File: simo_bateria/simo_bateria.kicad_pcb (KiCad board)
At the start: 2 copper layers, 65 x 35 mm, 16 parts, among them J1 BAT_LEVEL, J2 Plugin, J3 VBAT IN, J4 SWD, SW1 SW_Reed, U1 mod_mt3608, U2 BSS314PEH6327XTSA1

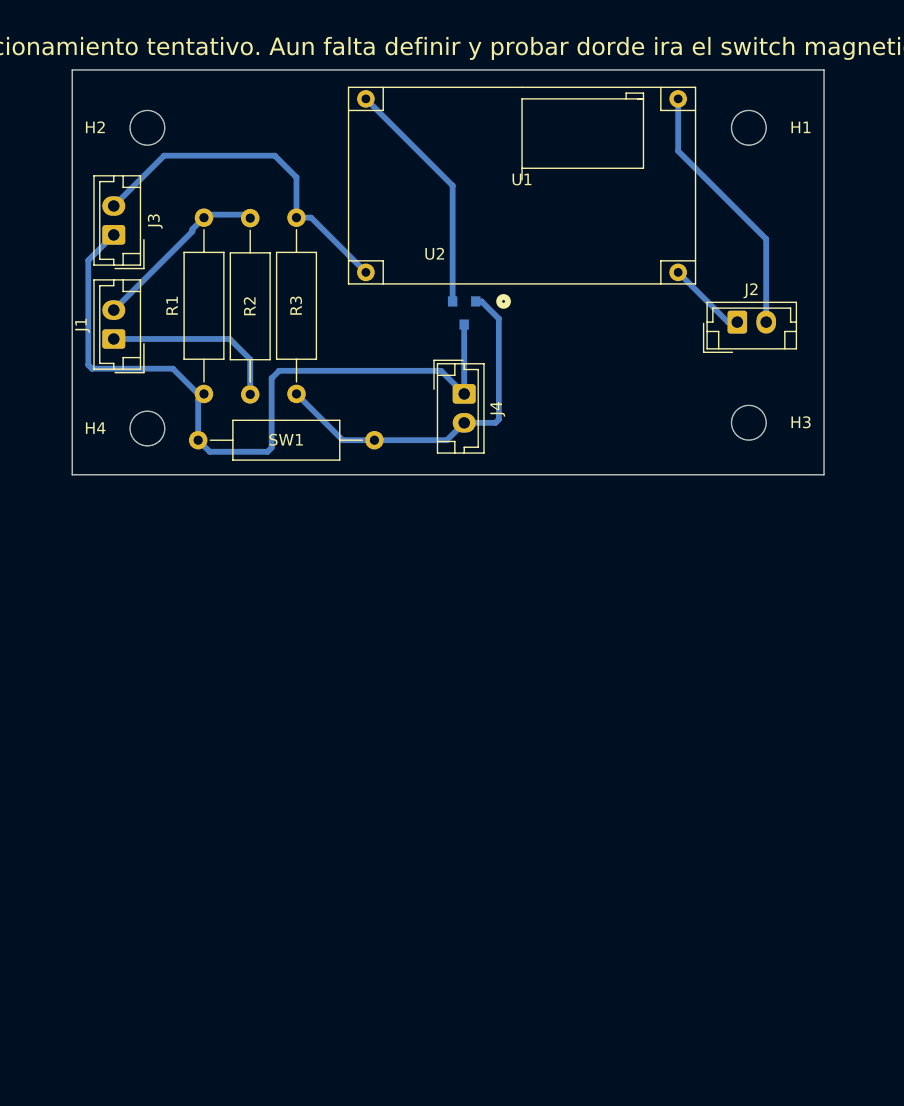
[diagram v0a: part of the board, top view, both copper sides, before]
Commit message: UPDATE
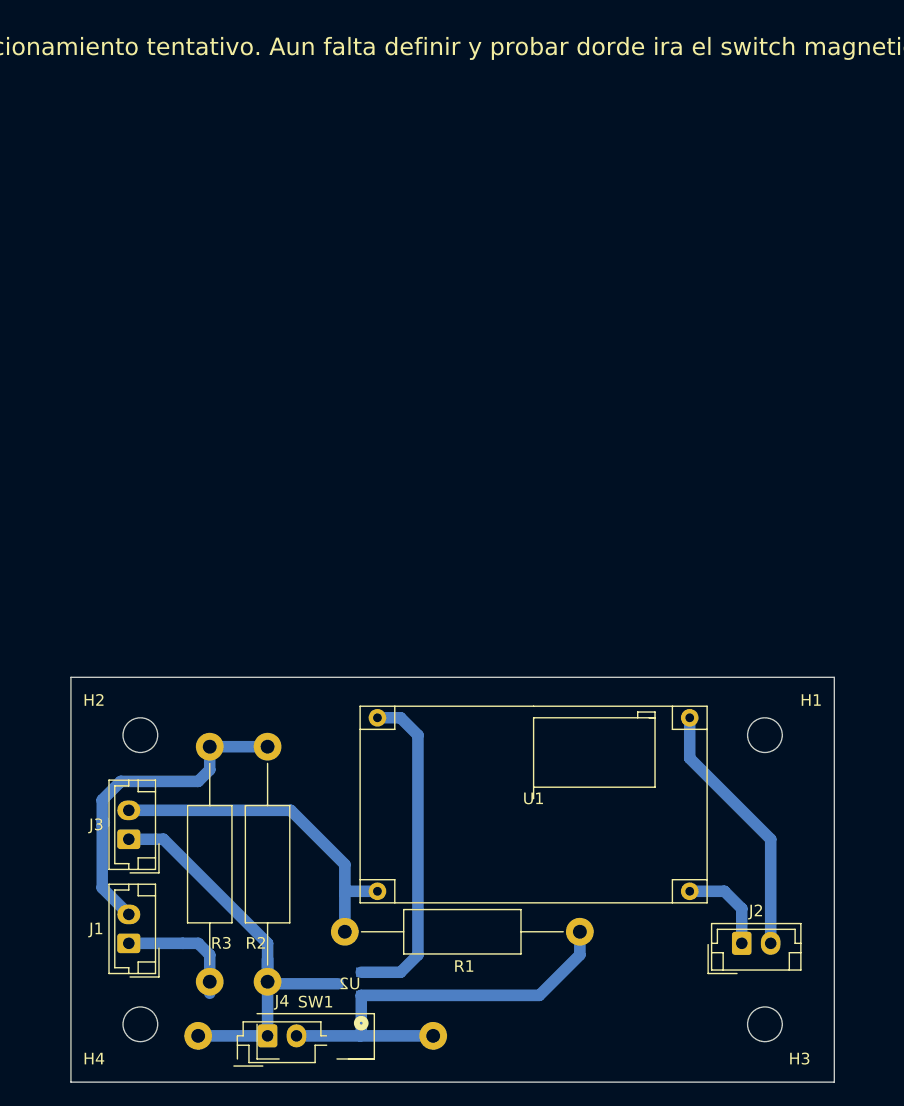
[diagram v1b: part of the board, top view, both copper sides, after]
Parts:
- R1: value 355k -> 10k; footprint Resistor_THT:R_Axial_DIN0309_L9.0mm_D3.2mm_P15.24mm_Horizontal -> simo_bateria:RESITOR_THT
- R2: value 155k -> 355k; footprint Resistor_THT:R_Axial_DIN0309_L9.0mm_D3.2mm_P15.24mm_Horizontal -> simo_bateria:RESITOR_THT
- R3: value 10k -> 155k; footprint Resistor_THT:R_Axial_DIN0309_L9.0mm_D3.2mm_P15.24mm_Horizontal -> simo_bateria:RESITOR_THT
- SW1: footprint Resistor_THT:R_Axial_DIN0309_L9.0mm_D3.2mm_P15.24mm_Horizontal -> simo_bateria:RESITOR_THT
- moved U2 58.8 mm to (179.1, 133.5), turned to 90 degrees
- moved J4 58.0 mm to (172.0, 138.0), turned to 0 degrees
- moved R1 56.7 mm to (199.0, 129.0), turned to 180 degrees
- moved J2 53.7 mm to (213.0, 130.0)
- moved U1 53.5 mm to (195.0, 118.0)
- moved H1 52.5 mm to (215.0, 112.0)
- moved H2 52.5 mm to (161.0, 112.0)
- moved J1 52.3 mm to (160.0, 130.0)
- moved J3 52.3 mm to (160.0, 121.0)
- moved H3 52.0 mm to (215.0, 137.0)
- moved H4 51.5 mm to (161.0, 137.0)
- moved SW1 51.5 mm to (166.0, 138.0)
- moved R2 45.7 mm to (172.0, 113.0)
- moved R3 31.4 mm to (167.0, 113.0), turned to -90 degrees
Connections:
- R1 pad 1: Net-(J3-Pad1) -> Net-(J4-Pad2)
- R1 pad 2: Net-(J1-Pad2) -> Net-(J3-Pad2)
- R2 pad 2: Net-(J1-Pad1) -> Net-(J3-Pad1)
- R3 pad 1: Net-(J4-Pad2) -> Net-(J1-Pad2)
- R3 pad 2: Net-(J3-Pad2) -> Net-(J1-Pad1)
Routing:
- net Net-(J3-Pad1): track 64.1 -> 36.0 mm
- net Net-(J1-Pad2): track 15.5 -> 28.4 mm
- net Net-(U1-Pad1): track 20.6 -> 28.6 mm
- net Net-(J4-Pad2): track 31.2 -> 37.7 mm
- net Net-(J1-Pad1): track 15.6 -> 10.7 mm
- net Net-(J2-Pad1): track 6.89 -> 8.12 mm
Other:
- board size 65 x 35 mm -> 66 x 35 mm
